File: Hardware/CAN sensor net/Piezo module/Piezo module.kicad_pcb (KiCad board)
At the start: 2 copper layers, 99.8 x 90.1 mm, 82 parts, among them J1 532610671, J2 532610671, J3 USB_B_Micro, J4 530470310, J5 532610271, SW1 SW_Push, SW2 SW_SPDT, U1 SN65HVD230, U2 STM32F103C8Tx, U3 W25Q32FVSSIG, U4 L78L05_SOT89, U5 LD3985M33R_SOT23, U6 L79L05_SOT89, U7 USBLC6-2SC6, U8 TL072, U9 ADS1120-PW, Y1 16MHz

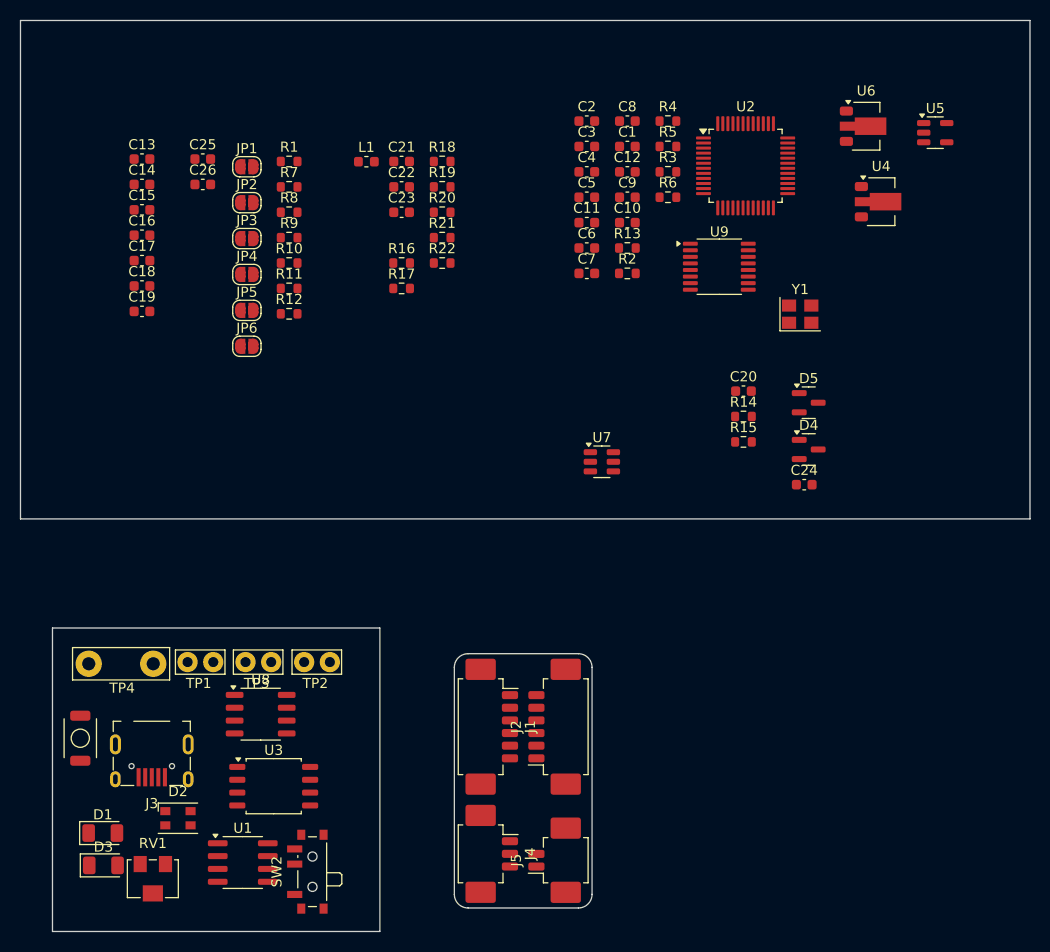
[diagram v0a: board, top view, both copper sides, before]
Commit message: Minor fixes
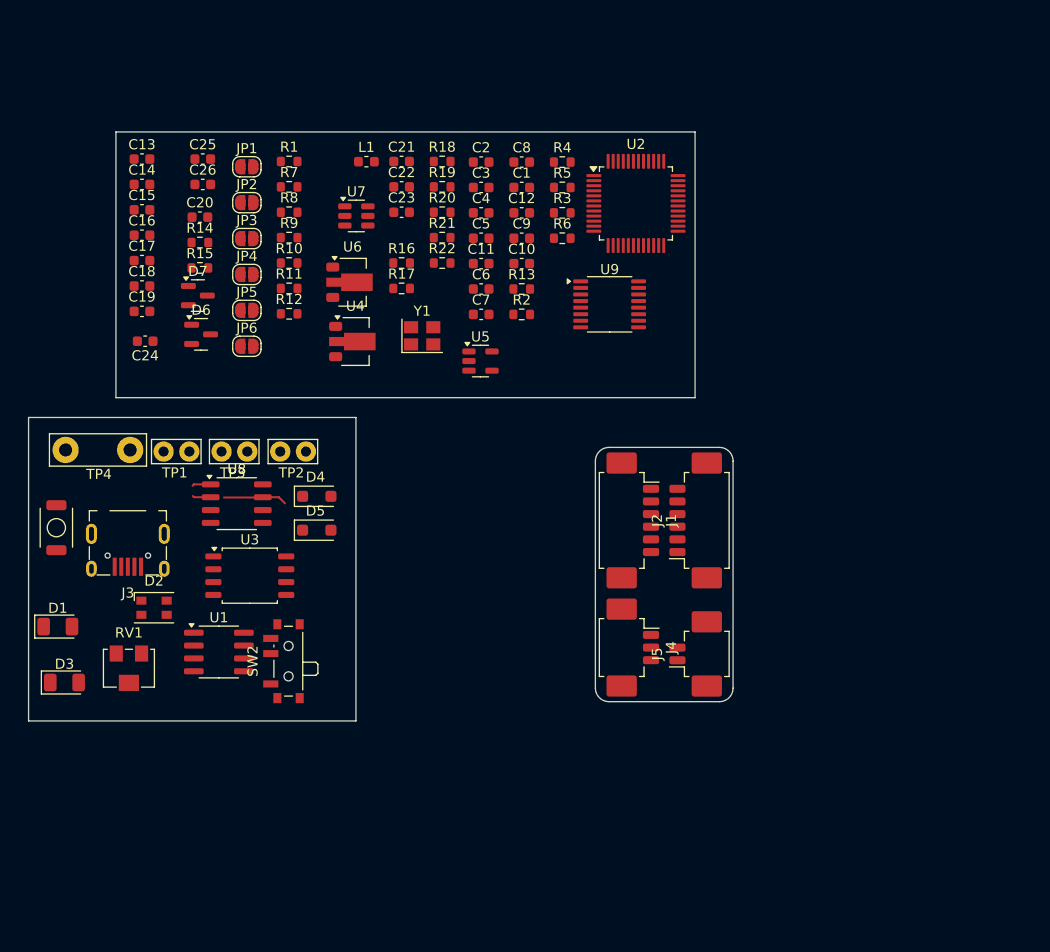
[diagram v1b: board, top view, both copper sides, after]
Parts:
- added D4: PMEG2020EH, Diode_SMD:D_SOD-123F, F.Cu at (87.3, 111.5)
- added D5: PMEG2020EH, Diode_SMD:D_SOD-123F, F.Cu at (87.3, 114.8)
- moved C24 66.7 mm to (70.3, 96.2), turned to 180 degrees
- moved D7 61.3 mm to (75.5, 91.6)
- moved D6 61.1 mm to (75.9, 95.5)
- moved R15 56.4 mm to (75.8, 88.9)
- moved C20 56.4 mm to (75.8, 83.9)
- moved R14 56.4 mm to (75.8, 86.4)
- moved U4 53.8 mm to (91.1, 96.2)
- moved U6 53.1 mm to (90.8, 90.3)
- moved U5 50.3 mm to (103.5, 98.1)
- moved Y1 37.4 mm to (97.7, 95.6)
- moved U7 34.4 mm to (91.2, 83.8)
- moved J4 24.7 mm to (118.0, 126.4)
- moved J5 24.7 mm to (125.4, 127.1)
- moved J1 24.7 mm to (118.0, 113.9)
- moved J2 24.7 mm to (125.4, 113.9)
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- renumbered D4 to D6, D5 to D7
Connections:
- C15 pad 1: VDD_7V0 -> Net-(D4-K)
- C15 pad 2: Net-(U5-GND) -> GND
- C16 pad 2: Net-(U5-GND) -> GND
- C19 pad 2: Net-(U5-GND) -> GND
- R16 pad 1: Net-(U8B-+) -> Net-(U8A-+)
- R17 pad 1: Net-(U8B-+) -> Net-(U8A-+)
- R20 pad 2: Net-(U8B--) -> Net-(U8A--)
- R21 pad 1: Net-(U8B--) -> Net-(U8A--)
- RV1 pad 2: Net-(U8A--) -> Net-(U8B--)
- U5 pad 1: VDD_7V0 -> Net-(D4-K)
- U5 pad 2: Net-(U5-GND) -> GND
- U5 pad 3: VDD_7V0 -> Net-(D4-K)
- U8 pad 1: Net-(R20-Pad1) -> Net-(R18-Pad1)
- U8 pad 3: GND -> Net-(U8A-+)
- U8 pad 5: Net-(U8B-+) -> GND
- U8 pad 7: Net-(R18-Pad1) -> Net-(R20-Pad1)
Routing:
- net Net-(R20-Pad1): track 0.00 -> 6.30 mm
- net Net-(R18-Pad1): track 0.00 -> 1.85 mm
- net Net-(U8A--): track 0.00 -> 1.82 mm
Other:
- board size 99.8 x 90.1 mm -> 69.7 x 58.2 mm
- board text added: "CAN"
- board text added: "PWR"
